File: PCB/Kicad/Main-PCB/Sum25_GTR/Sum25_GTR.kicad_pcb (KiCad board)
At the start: 2 copper layers, 182 x 48 mm, 20 parts, among them J3 IDC_5x2, U4 DRV5055A2xLPGxQ1, U5 DRV5055A2xLPGxQ1

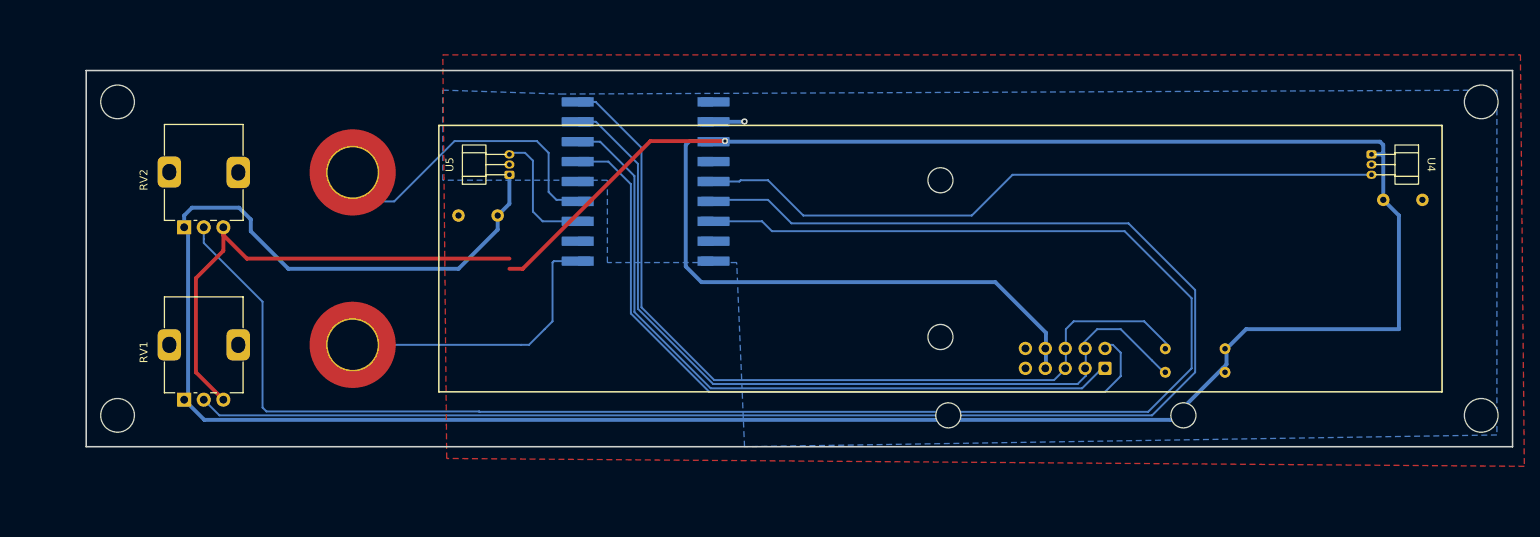
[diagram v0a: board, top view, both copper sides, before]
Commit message: update all kicad designs for week 1
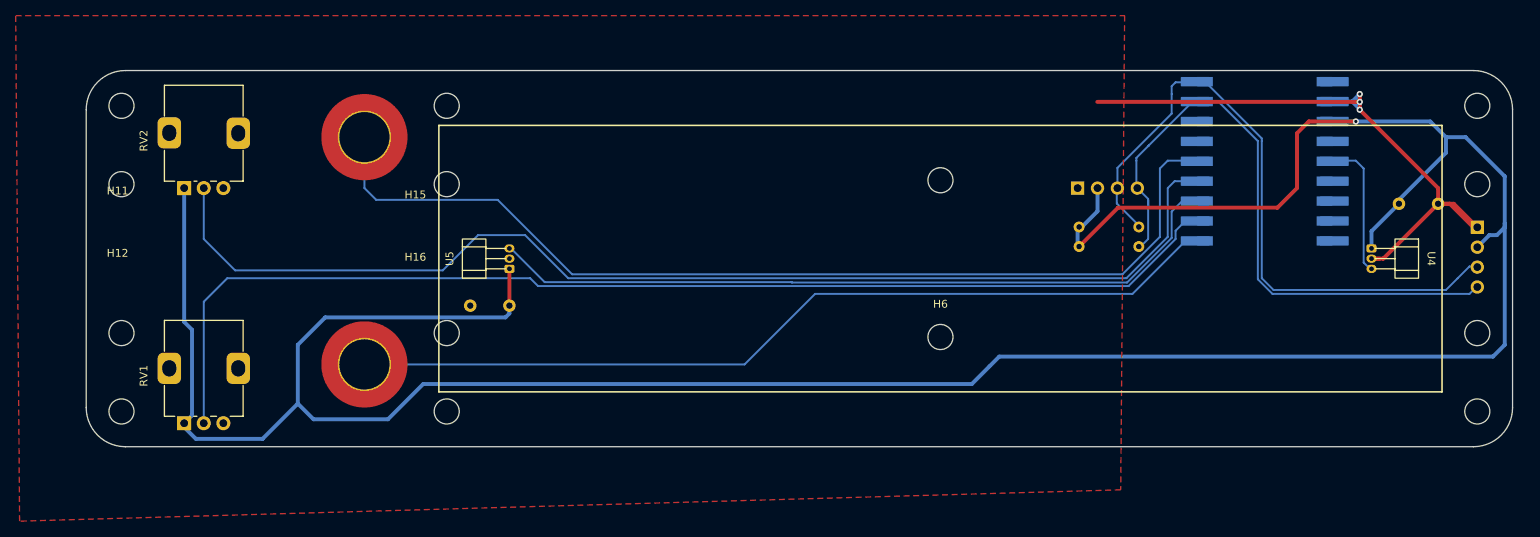
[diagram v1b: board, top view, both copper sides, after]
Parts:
- removed J3: IDC_5x2, Connector_IDC:IDC-Header_2x05_P2.54mm_Vertical
- added H11: MountingHole, MountingHole:MountingHole_3.2mm_M3, F.Cu at (48.0, 89.5)
- added H12: MountingHole, MountingHole:MountingHole_3.2mm_M3, F.Cu at (48.0, 97.5)
- added H13: MountingHole, MountingHole:MountingHole_3.2mm_M3, F.Cu at (222.0, 104.5)
- added H14: MountingHole, MountingHole:MountingHole_3.2mm_M3, F.Cu at (221.0, 85.0)
- added H15: MountingHole, MountingHole:MountingHole_3.2mm_M3, F.Cu at (86.0, 90.0)
- added H16: MountingHole, MountingHole:MountingHole_3.2mm_M3, F.Cu at (86.0, 98.0)
- added J1: Conn_01x04_Pin, Connector_PinSocket_2.54mm:PinSocket_1x04_P2.54mm_Vertical, B.Cu at (221.5, 90.0)
- added J2: Conn_01x04_Pin, Connector_PinSocket_2.54mm:PinSocket_1x04_P2.54mm_Vertical, B.Cu at (170.5, 85.0)
- H1, H2, H3, H5: footprint MountingHole:MountingHole_4.3mm_M4 -> MountingHole:MountingHole_3.2mm_M3
- moved H10 102.8 mm to (90.5, 73.5)
- moved U2 79.0 mm to (194.4, 81.6)
- moved H6 72.3 mm to (153.0, 104.0)
- moved H9 65.5 mm to (88.5, 114.5)
- moved H3 33.0 mm to (221.5, 73.0)
- moved R2 24.6 mm to (170.7, 92.5), turned to 0 degrees
- moved R3 24.3 mm to (170.7, 90.0), turned to 0 degrees
- moved U4 12.0 mm to (208.0, 94.0)
- moved U5 12.0 mm to (98.0, 94.0)
- moved C4 11.6 mm to (98.0, 100.0)
- moved RV2 5.00 mm to (56.5, 85.0)
- moved H7 4.74 mm to (79.5, 78.5)
- moved RV1 3.00 mm to (56.5, 115.0)
- moved H8 2.92 mm to (79.5, 107.5)
- moved C3 2.06 mm to (211.5, 87.0)
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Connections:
- H7 pad 1: /A9 -> /D0
- RV1 pad 2: /A2 -> /A7
- RV2 pad 2: /A3 -> /A9
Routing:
- net /A3: track 222.2 -> 0.00 mm
- net /A2: track 206.4 -> 0.00 mm
- net /A7: track 0.00 -> 148.8 mm
- net /D0: track 0.00 -> 130.0 mm
- net /A9: track 40.3 -> 149.8 mm
- net /D1: track 96.2 -> 0.00 mm
- net /D2: track 90.8 -> 0.00 mm
- net +3.3V: track 461.3 -> 374.5 mm
- net /A8: track 17.2 -> 97.1 mm
- net /A6: track 38.6 -> 113.4 mm
- net /A1: track 89.1 -> 17.2 mm
- net /SCL: track 108.2 -> 82.8 mm
- net /SDA: track 106.5 -> 82.7 mm
- net GND: track 68.7 -> 85.8 mm, vias 1 -> 3
- removed copper zone on B.Cu, net GND
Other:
- outline, holes or cut-outs redrawn
- board text added: "0.1uF"
- board text added: "2.2k"
- board text added: "Creativitas Barre v2"
- board text removed: "Creativitas Barré v1"
- board text removed: "IRQ"
